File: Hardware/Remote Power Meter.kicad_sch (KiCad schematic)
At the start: 33 parts, among them J1 USB_C_Receptacle_USB2.0, J2 Conn_01x04_Female, J3 Conn_01x04_Male, J4 Conn_01x02, J5 USB_A, J6 Conn_01x02, Q1 UMH3N, SW1 SW_Push, U1 AMS1117-3.3, U2 INA219AxD, U3 CH340C

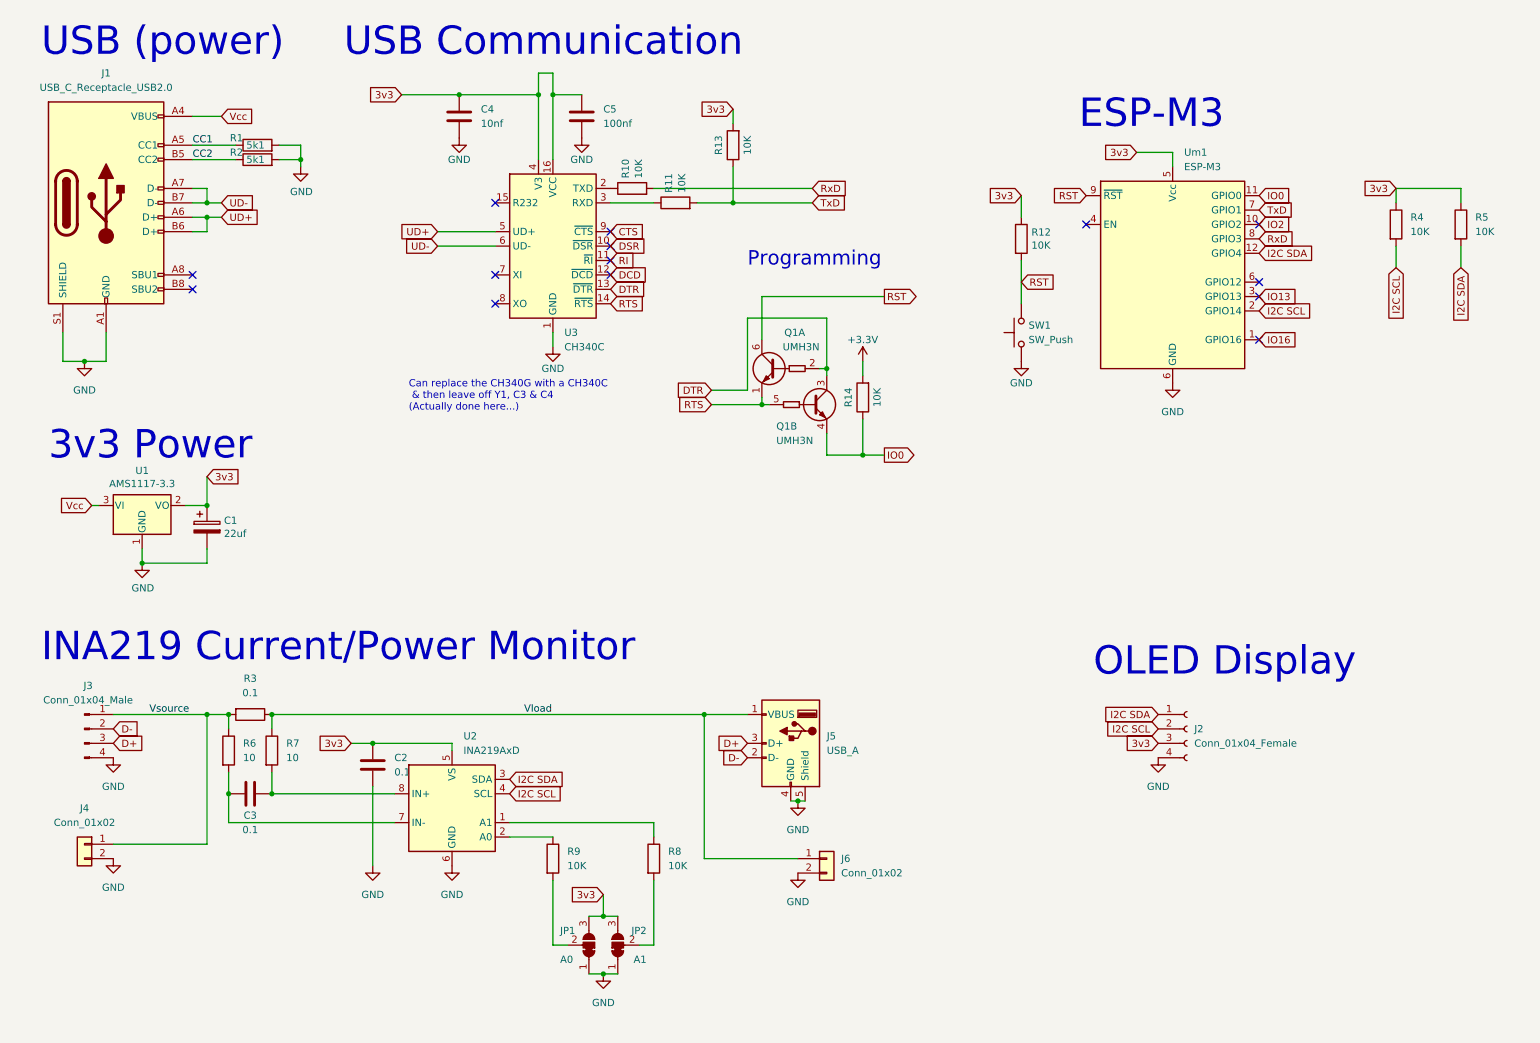
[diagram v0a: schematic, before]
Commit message: Possibly reached v1.0.0
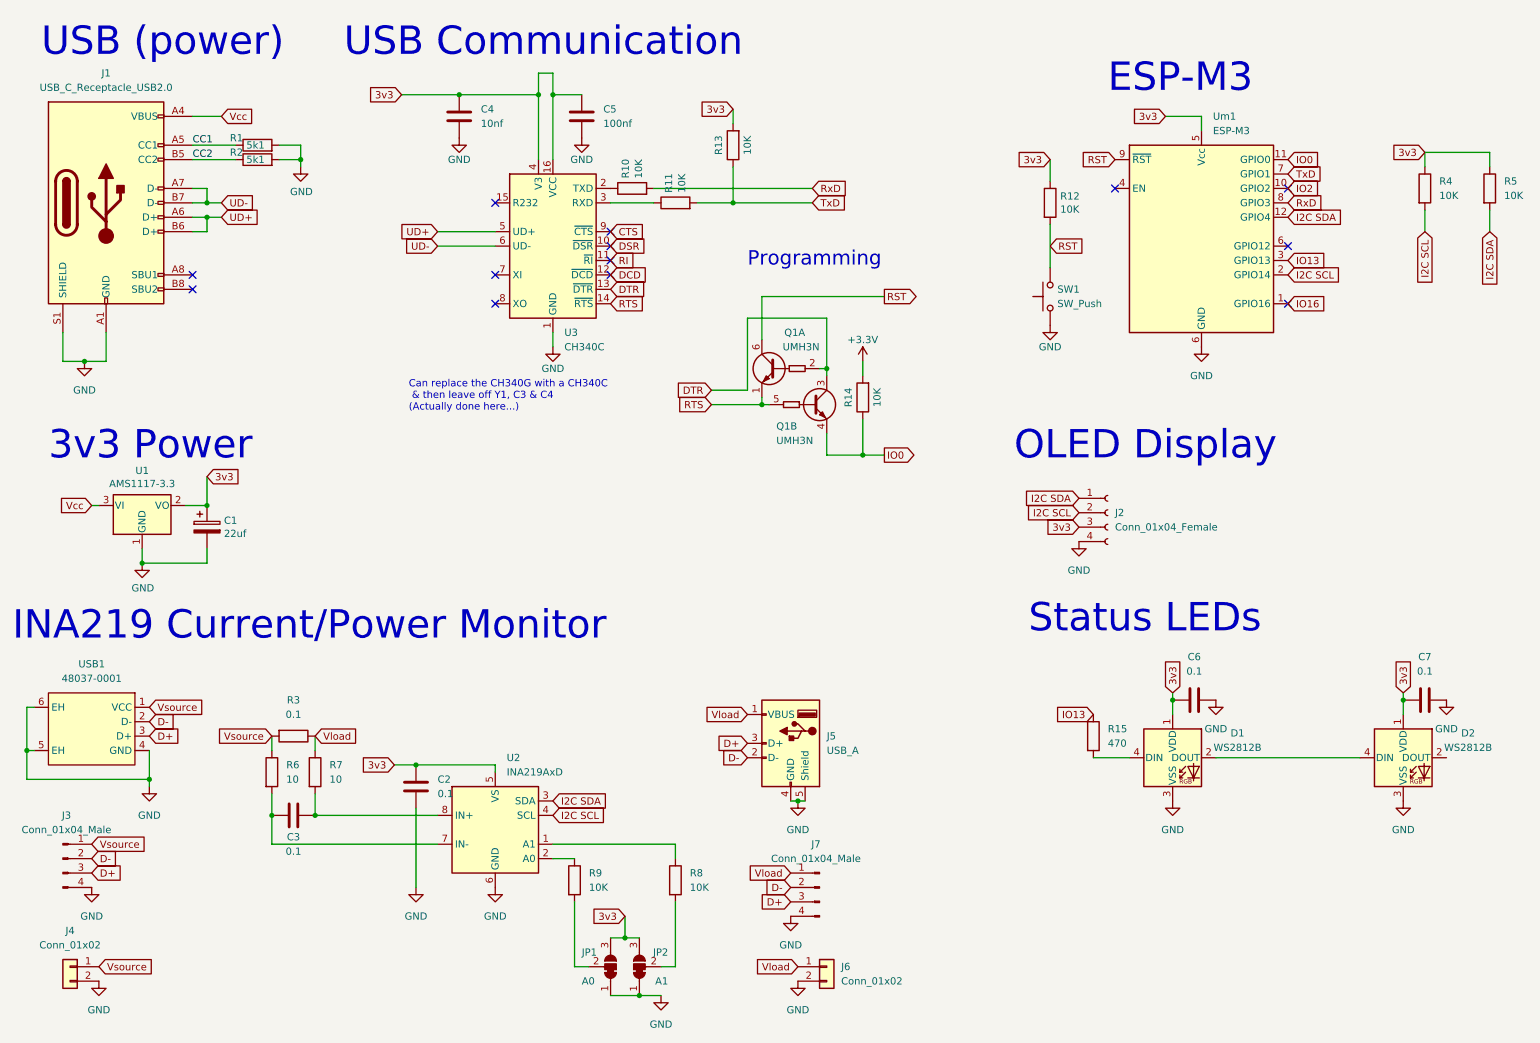
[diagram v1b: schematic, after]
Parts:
- added C6, C7: 0.1, Capacitor_SMD:C_0603_1608Metric_Pad1.08x0.95mm_HandSolder, symbol Device:C
- added D1, D2: WS2812B, LED_SMD:LED_WS2812B_PLCC4_5.0x5.0mm_P3.2mm, symbol LED:WS2812B
- added J7: Conn_01x04_Male, Connector_PinHeader_2.54mm:PinHeader_1x04_P2.54mm_Vertical, symbol Connector:Conn_01x04_Male
- added R15: 470, Resistor_SMD:R_0603_1608Metric_Pad0.98x0.95mm_HandSolder, symbol Device:R
- added USB1: 48037-0001, Tinker:USB-A-TH_48037-0001, symbol USB-A-TH_48037-0001:48037-0001
- J3: footprint Connector_PinHeader_2.54mm:PinHeader_1x04_P2.54mm_Horizontal -> Connector_PinHeader_2.54mm:PinHeader_1x04_P2.54mm_Vertical
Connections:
- net 3v3: now also C6.1, C7.1, D1.1 (VDD), D2.1 (VDD)
- net D+: now also J7.3 (Pin_3), USB1.3 (D+)
- net D-: now also J7.2 (Pin_2), USB1.2 (D-)
- net GND: now also C6.2, C7.2, D1.3 (VSS), D2.3 (VSS), J7.4 (Pin_4), USB1.4 (GND), USB1.5 (EH), USB1.6 (EH)
- net IO13: now also R15.1
- net Vload: now also J7.1 (Pin_1)
- net Vsource: now also USB1.1 (VCC)
- new net: D1.2 (DOUT), D2.4 (DIN)
- new net: D1.4 (DIN), R15.2
- no-connect marks 14 -> 13
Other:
- note added: "Status LEDs"
- moved on the sheet: C2, C3, J2, J3, J4, J6, JP1, JP2, R12, R3, R4, R5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
